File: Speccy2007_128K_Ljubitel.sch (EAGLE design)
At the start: 112 parts, among them X1 5V, X2 SCART-F, X3 PS/2 KB, X4 SD Card, X5 ByteBlaster, X6 AVRISP

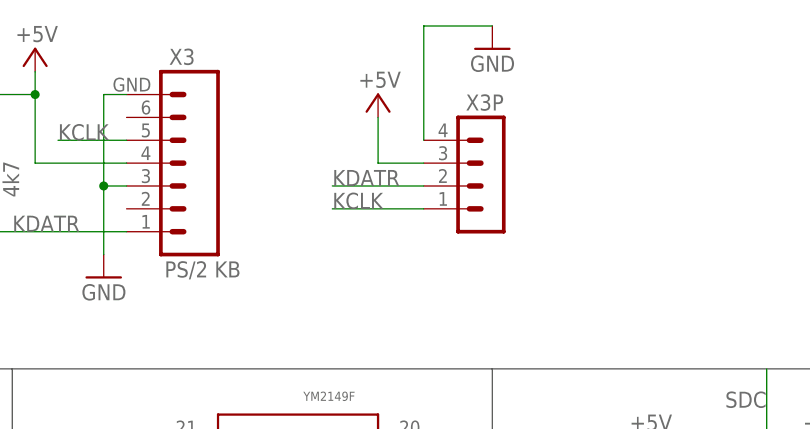
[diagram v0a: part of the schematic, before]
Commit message: .
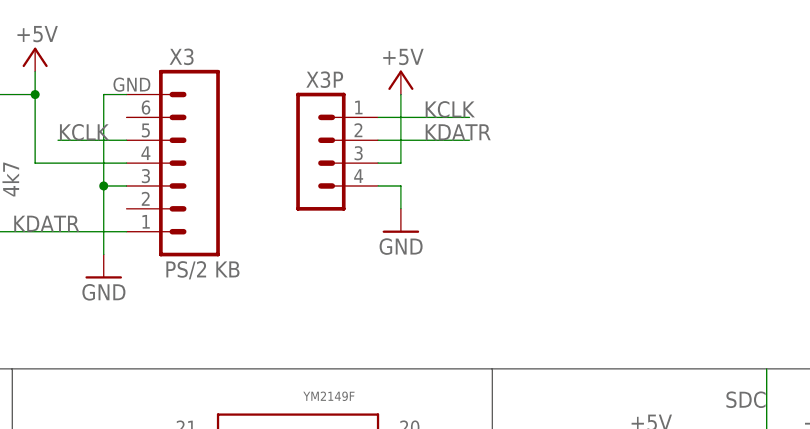
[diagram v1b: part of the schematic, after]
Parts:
- R2: device rcl:R-EU_M1206 -> rcl:R-EU_R1206
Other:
- moved on the sheet: X3P
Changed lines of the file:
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@@
 <part name="R9P2" library="rcl" deviceset="R-EU_" device="R1206" value="75"/>
 <part name="J1" library="rcl" deviceset="R-EU_" device="M1206"/>
-<part name="R2" library="rcl" deviceset="R-EU_" device="M1206"/>
+<part name="R2" library="rcl" deviceset="R-EU_" device="R1206"/>
 <part name="DD12" library="Speccy" deviceset="74*74" device="O" technology="LS" value="74LS74O"/>
 <part name="P+15" library="supply1" deviceset="+5V" device=""/>
@@
 <instance part="CP2" gate="G$1" x="121.92" y="231.14"/>
 <instance part="CP1" gate="G$1" x="111.76" y="231.14"/>
-<instance part="X3P" gate="1" x="297.18" y="233.68" rot="MR0"/>
-<instance part="P+17" gate="1" x="284.48" y="241.3" smashed="yes">
-<attribute name="VALUE" x="287.02" y="243.84" size="1.778" layer="96" rot="R180"/>
+<instance part="X3P" gate="1" x="276.86" y="233.68" smashed="yes" rot="MR180">
+<attribute name="VALUE" x="275.59" y="243.84" size="1.778" layer="96" rot="MR180"/>
+<attribute name="NAME" x="280.67" y="242.062" size="1.778" layer="95" rot="MR0"/>
 </instance>
-<instance part="GND29" gate="1" x="297.18" y="246.38" rot="MR0"/>
+<instance part="P+17" gate="1" x="287.02" y="243.84" smashed="yes">
+<attribute name="VALUE" x="289.56" y="246.38" size="1.778" layer="96" rot="R180"/>
+</instance>
+<instance part="GND29" gate="1" x="287.02" y="226.06" rot="MR0"/>
 </instances>
 <busses>
@@
 <segment>
 <pinref part="X3P" gate="1" pin="4"/>
-<wire x1="289.56" y1="236.22" x2="289.56" y2="248.92" width="0.1524" layer="91"/>
 <pinref part="GND29" gate="1" pin="GND"/>
-<wire x1="289.56" y1="248.92" x2="297.18" y2="248.92" width="0.1524" layer="91"/>
+<wire x1="284.48" y1="231.14" x2="287.02" y2="231.14" width="0.1524" layer="91"/>
+<wire x1="287.02" y1="231.14" x2="287.02" y2="228.6" width="0.1524" layer="91"/>
 </segment>
 </net>
@@
 <pinref part="P+17" gate="1" pin="+5V"/>
 <pinref part="X3P" gate="1" pin="3"/>
-<wire x1="289.56" y1="233.68" x2="284.48" y2="233.68" width="0.1524" layer="91"/>
-<wire x1="284.48" y1="233.68" x2="284.48" y2="238.76" width="0.1524" layer="91"/>
+<wire x1="284.48" y1="233.68" x2="287.02" y2="233.68" width="0.1524" layer="91"/>
+<wire x1="287.02" y1="233.68" x2="287.02" y2="241.3" width="0.1524" layer="91"/>
 </segment>
 </net>
@@
 </segment>
 <segment>
-<label x="279.4" y="228.6" size="1.778" layer="95"/>
-<wire x1="289.56" y1="228.6" x2="279.4" y2="228.6" width="0.1524" layer="91"/>
+<label x="289.56" y="238.76" size="1.778" layer="95"/>
+<wire x1="284.48" y1="238.76" x2="294.64" y2="238.76" width="0.1524" layer="91"/>
 <pinref part="X3P" gate="1" pin="1"/>
 </segment>
@@
 </segment>
 <segment>
-<label x="279.4" y="231.14" size="1.778" layer="95"/>
-<wire x1="289.56" y1="231.14" x2="279.4" y2="231.14" width="0.1524" layer="91"/>
+<label x="289.56" y="236.22" size="1.778" layer="95"/>
+<wire x1="284.48" y1="236.22" x2="294.64" y2="236.22" width="0.1524" layer="91"/>
 <pinref part="X3P" gate="1" pin="2"/>
 </segment>

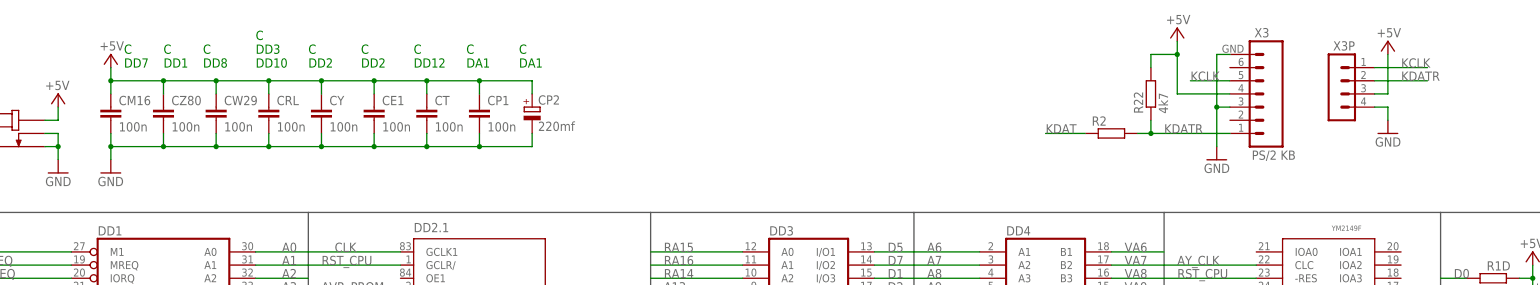
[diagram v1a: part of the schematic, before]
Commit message: .
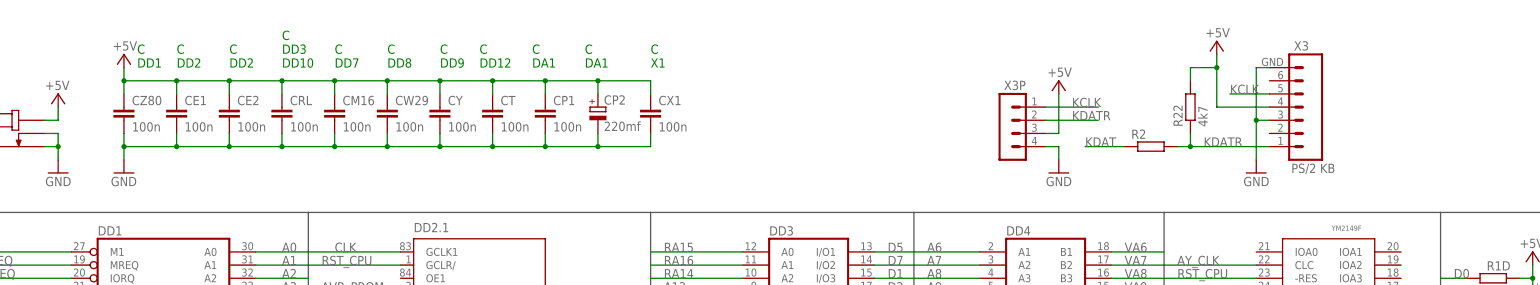
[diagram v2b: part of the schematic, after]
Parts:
- added CE2, CX1: 100n, rcl:C-EUC0805
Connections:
- net +5V: now also CE2.1, CX1.1
- net GND: now also CE2.2, CX1.2
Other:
- note added: "C DD9"
- note added: "C X1"
- moved on the sheet: CE1, CM16, CP1, CP2, CRL, CT, CW29, CY, CZ80, R2, R22, X3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
